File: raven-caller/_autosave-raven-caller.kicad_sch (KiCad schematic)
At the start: 14 parts, among them J1 I2C LCD, J2 Conn_Coaxial, Q1 BSS138, SW1 RotaryEncoder_Switch, U1 SeeeduinoXIAO, U2 RFM95W-915S2, U3 24LC256, U4 PCF8574AP

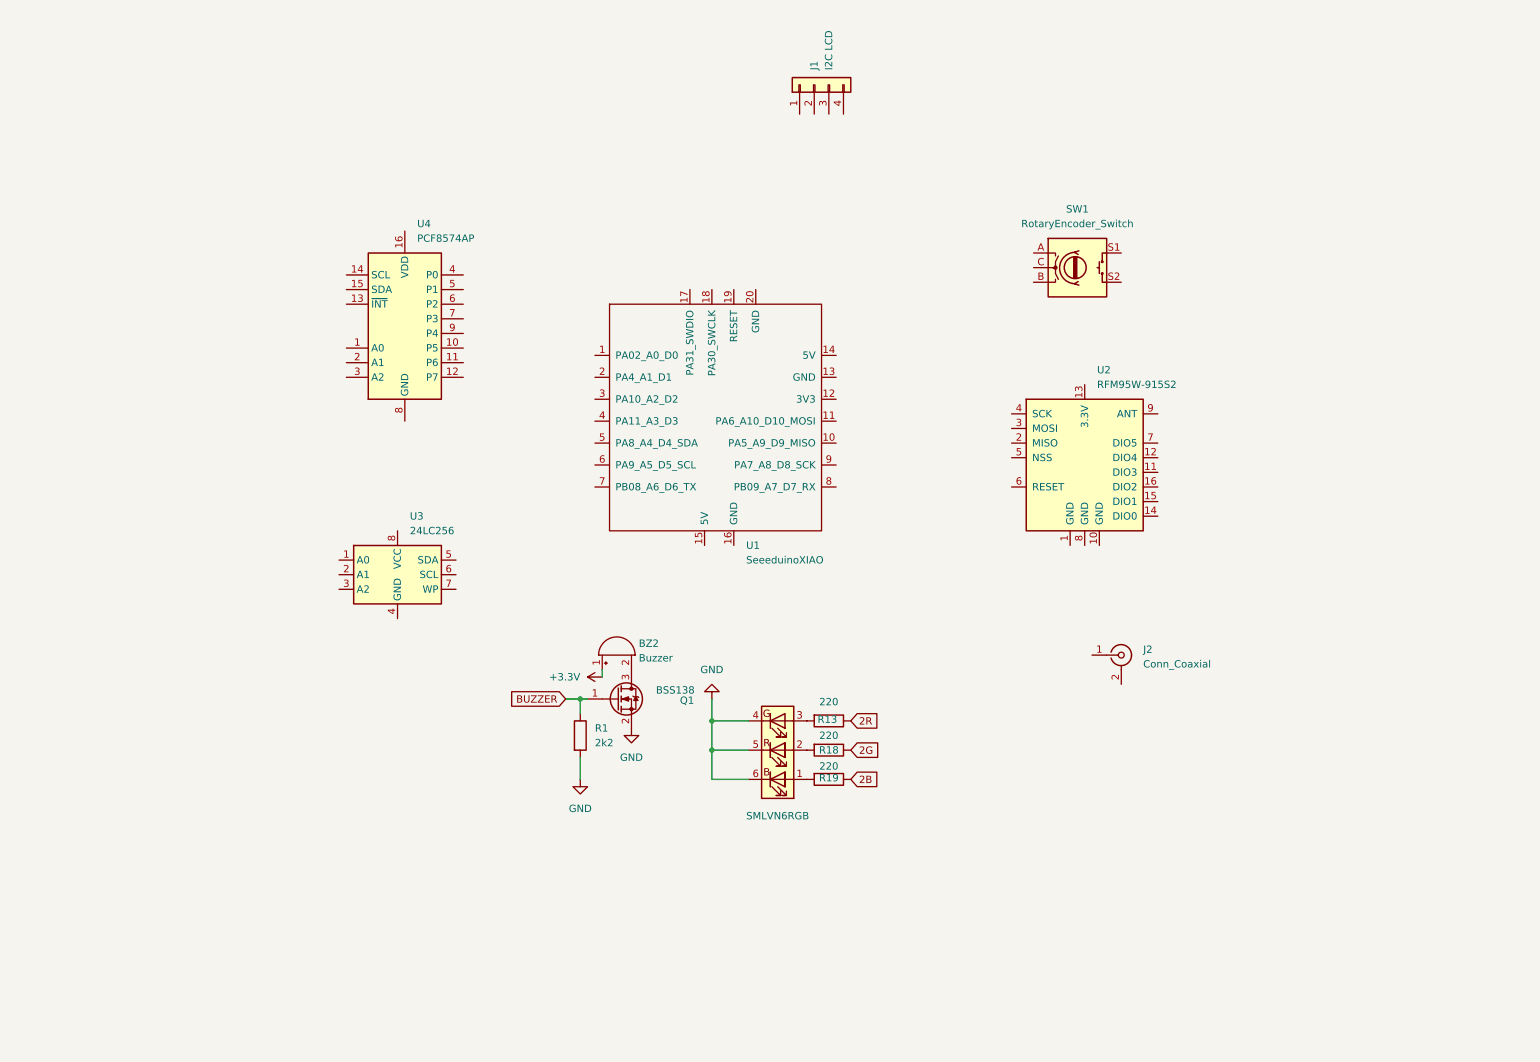
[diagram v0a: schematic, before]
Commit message: schematic v1 done
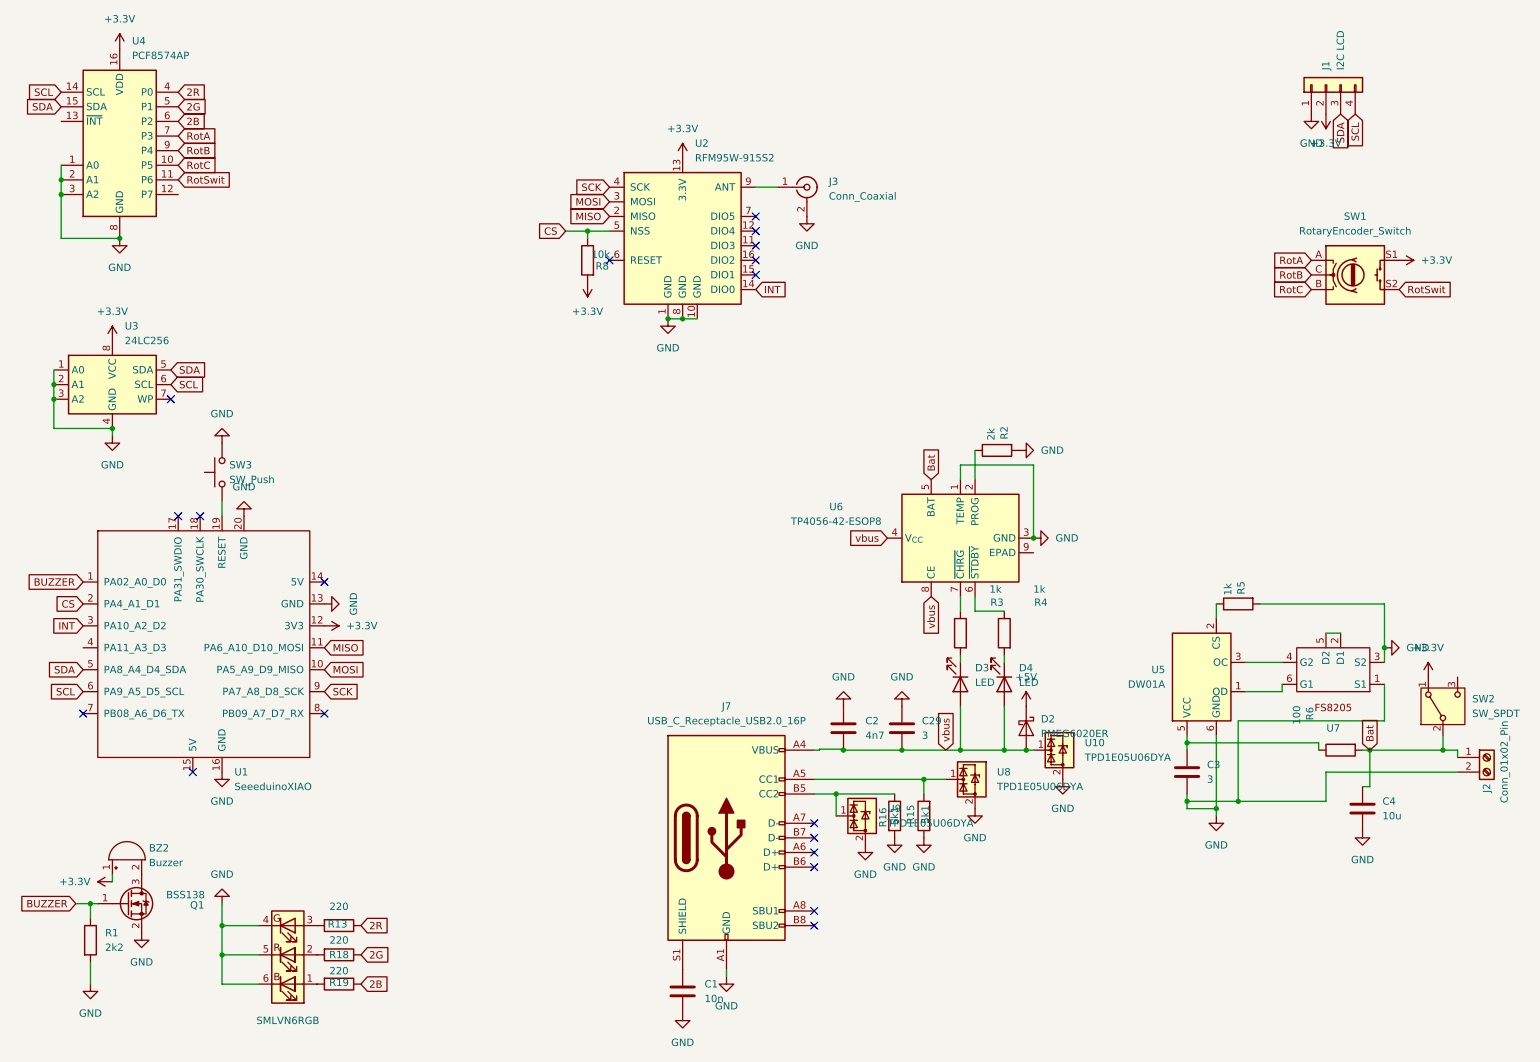
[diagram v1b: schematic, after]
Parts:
- removed J2: Conn_Coaxial, Connector_Coaxial:SMA_Amphenol_901-143_Horizontal, symbol Connector:Conn_Coaxial
- added C1: 10n, Capacitor_SMD:C_0603_1608Metric, symbol Device:C
- added C2: 4n7, Capacitor_SMD:C_0603_1608Metric, symbol Device:C
- added C29, C3: 3, Capacitor_SMD:C_0603_1608Metric, symbol Device:C
- added C4: 10u, Capacitor_SMD:C_0603_1608Metric, symbol Device:C
- added D2: PMEG6020ER, Diode_SMD:Nexperia_CFP3_SOD-123W, symbol Diode:PMEG6020ER
- added D3, D4: LED, LED_SMD:LED_0603_1608Metric, symbol Device:LED
- added J2: Conn_01x02_Pin, Connector_JST:JST_PH_B2B-PH-K_1x02_P2.00mm_Vertical, symbol Connector:Screw_Terminal_01x02
- added J3: Conn_Coaxial, Connector_Coaxial:U.FL_Molex_MCRF_73412-0110_Vertical, symbol Connector:Conn_Coaxial
- added J7: USB_C_Receptacle_USB2.0_16P, Connector_USB:USB_C_Receptacle_GCT_USB4105-xx-A_16P_TopMnt_Horizontal, symbol Connector:USB_C_Receptacle_USB2.0_16P
- added R15, R16: 5k1, Resistor_SMD:R_0603_1608Metric, symbol Device:R
- added R2: 2k, Resistor_SMD:R_0603_1608Metric, symbol Device:R
- added R3, R4, R5: 1k, Resistor_SMD:R_0603_1608Metric, symbol Device:R
- added R6: 100, Resistor_SMD:R_0603_1608Metric, symbol Device:R
- added R8: 10k, Resistor_SMD:R_0603_1608Metric, symbol Device:R
- added SW2: SW_SPDT, Button_Switch_THT:SW_Slide_SPDT_Angled_CK_OS102011MA1Q, symbol Switch:SW_SPDT
- added SW3: SW_Push, Button_Switch_THT:SW_PUSH_6mm, symbol Switch:SW_Push
- added U10, U8, U9: TPD1E05U06DYA, Diode_SMD:D_SOD-523, symbol Power_Protection:TPD1E05U06DYA
- added U5: DW01A, Package_TO_SOT_SMD:SOT-23-6, symbol Battery_Management:DW01A
- added U6: TP4056-42-ESOP8, Package_SO:SOIC-8-1EP_3.9x4.9mm_P1.27mm_EP2.41x3.3mm_ThermalVias, symbol Battery_Management:TP4056-42-ESOP8
- added U7: ~, Package_TO_SOT_SMD:SOT-23-6, symbol FS8205:FS8205
- J1: footprint (none) -> Connector_PinHeader_2.54mm:PinHeader_1x04_P2.54mm_Horizontal
- SW1: footprint (none) -> Rotary_Encoder:RotaryEncoder_Alps_EC11E-Switch_Vertical_H20mm
- U1: footprint (none) -> Xiao Seeed SAMD21:XiaoSeeed
- U3: footprint (none) -> Package_SO:SOIC-8_3.9x4.9mm_P1.27mm
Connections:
- net +3.3V: now also J1.2 (Pin_2), SW1.S1, U1.12 (3V3), U2.13 (3.3V), U3.8 (VCC), U4.16 (VDD), R8.2, SW2.1 (A)
- net 2B: now also U4.6 (P2)
- net 2G: now also U4.5 (P1)
- net 2R: now also U4.4 (P0)
- net BUZZER: now also U1.1 (PA02_A0_D0)
- net GND: now also J1.1 (Pin_1), U1.13 (GND), U1.16 (GND), U1.20 (GND), U2.1 (GND), U2.10 (GND), U2.8 (GND), U3.1 (A0), U3.2 (A1), U3.3 (A2), U3.4 (GND), U4.1 (A0), U4.2 (A1), U4.3 (A2), U4.8 (GND), C1.2, C2.1, C29.1, C3.2, C4.2, J2.2 (Pin_2), J3.2 (Ext), J7.A1 (GND), J7.A12 (GND), J7.B1 (GND), J7.B12 (GND), R15.1, R16.2, R2.2, R5.2, SW3.2, U10.2 (GND), U5.6 (GND), U6.1 (TEMP), U6.3 (GND), U7.1 (S1), U7.3 (S2), U8.2 (GND), U9.2 (GND)
- net INT: now reaches U2.14 (DIO0)
- net INT: now also U1.3 (PA10_A2_D2)
- net MISO: now reaches U2.2 (MISO)
- net MISO: now also U1.11 (PA6_A10_D10_MOSI)
- net MOSI: now reaches U2.3 (MOSI)
- net MOSI: now also U1.10 (PA5_A9_D9_MISO)
- net SCK: now reaches U2.4 (SCK)
- net SCK: now also U1.9 (PA7_A8_D8_SCK)
- net CS: now reaches U2.5 (NSS)
- net CS: now also U1.2 (PA4_A1_D1), R8.1
- net at U2.9 (ANT): now also J3.1 (In)
- net SDA: now reaches U3.5 (SDA)
- net SDA: now also J1.3 (Pin_3), U1.5 (PA8_A4_D4_SDA), U4.15 (SDA)
- net SCL: now reaches U3.6 (SCL)
- net SCL: now also J1.4 (Pin_4), U1.6 (PA9_A5_D5_SCL), U4.14 (SCL)
- net RotA: now reaches SW1.A
- net RotA: now also U4.7 (P3)
- net RotC: now reaches SW1.B
- net RotC: now also U4.10 (P5)
- net RotB: now reaches SW1.C
- net RotB: now also U4.9 (P4)
- net RotSwit: now reaches SW1.S2
- net RotSwit: now also U4.11 (P6)
- net at U1.19 (RESET): now also SW3.1
- new net: U7.2 (D1), U7.5 (D2)
- new net: U5.3 (OC), U7.4 (G2)
- new net: U5.1 (OD), U7.6 (G1)
- new net: C3.1, R6.1, U5.5 (VCC)
- new net: J7.A5 (CC1), R15.2, U8.1 (I/O)
- new net: D3.1 (K), R3.2
- new net: R3.1, U6.7 (~{CHRG})
- new net: R5.1, U5.2 (CS)
- new net: D4.1 (K), R4.2
- new net: R4.1, U6.6 (~{STDBY})
- new net: J7.B5 (CC2), R16.1, U9.1 (I/O)
- new net: C1.1, J7.S1 (SHIELD)
- new net: R2.1, U6.2 (PROG)
- new net +5V: D2.1 (K)
- new net Bat: C4.1, J2.1 (Pin_1), R6.2, SW2.2 (B), U6.5 (BAT)
- new net vbus: C2.2, C29.2, D2.2 (A), D3.2 (A), D4.2 (A), J7.A4 (VBUS), J7.A9 (VBUS), J7.B4 (VBUS), J7.B9 (VBUS), U10.1 (I/O), U6.4 (V_{CC}), U6.8 (CE)
- no-connect marks 0 -> 19
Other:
- moved on the sheet: BZ2, J1, Q1, R1, R13, R18, R19, SW1, U1, U2, U3, U4
